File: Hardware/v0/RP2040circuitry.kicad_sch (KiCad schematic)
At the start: 29 parts, among them J1 TYPE-C-31-M-12, SW1 SW_Push, U1 RP2040, U2 NCP1117-3.3_SOT223, U3 W25Q128JVS, X1 ABM8-272-T3

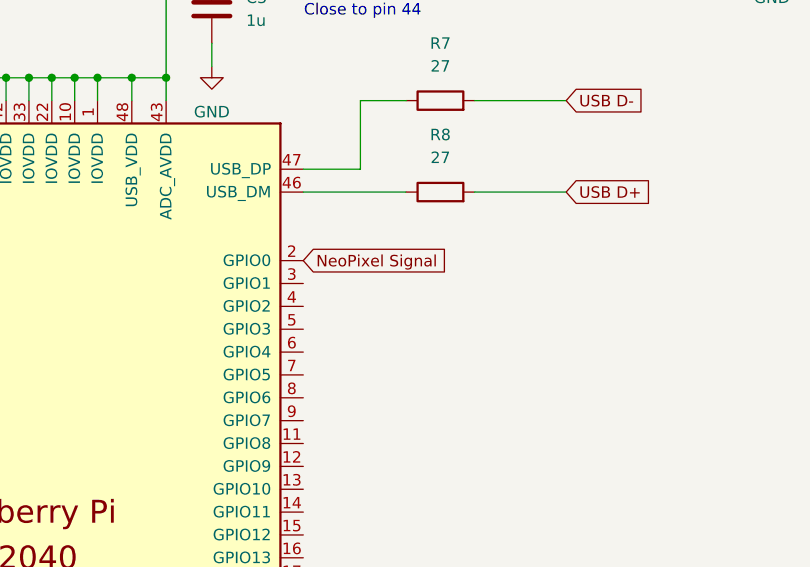
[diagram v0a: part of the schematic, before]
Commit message: he
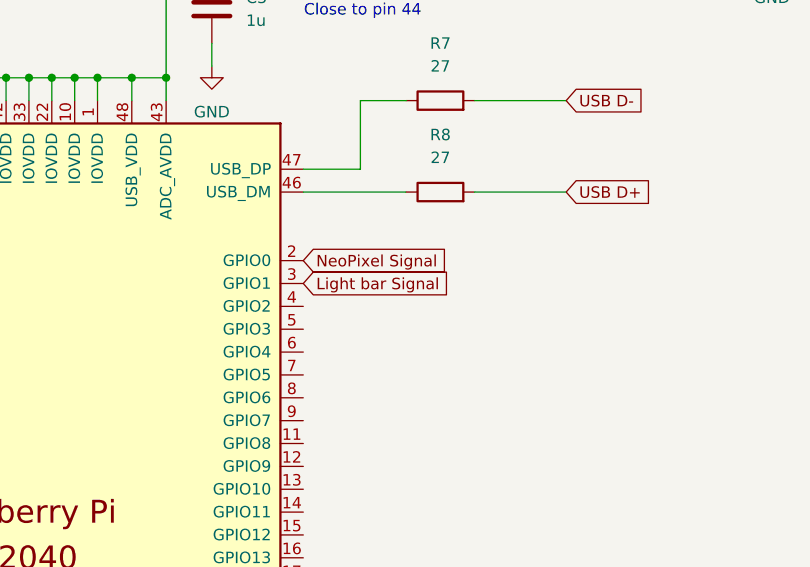
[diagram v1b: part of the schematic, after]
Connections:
- net Light bar Signal: now reaches U1.3 (GPIO1)
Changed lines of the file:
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@@
+		)
+	)
+	(global_label "Light bar Signal"
+		(shape input)
+		(at 238.76 78.74 0)
+		(fields_autoplaced yes)
+		(effects
+			(font
+				(size 1.27 1.27)
+			)
+			(justify left)
+		)
+		(property "Intersheetrefs" "${INTERSHEET_REFS}"
+			(at 257.3477 78.74 0)
+			(effects
+				(font
+					(size 1.27 1.27)
+				)
+				(justify left)
+				(hide yes)
+			)
 		)
 	)

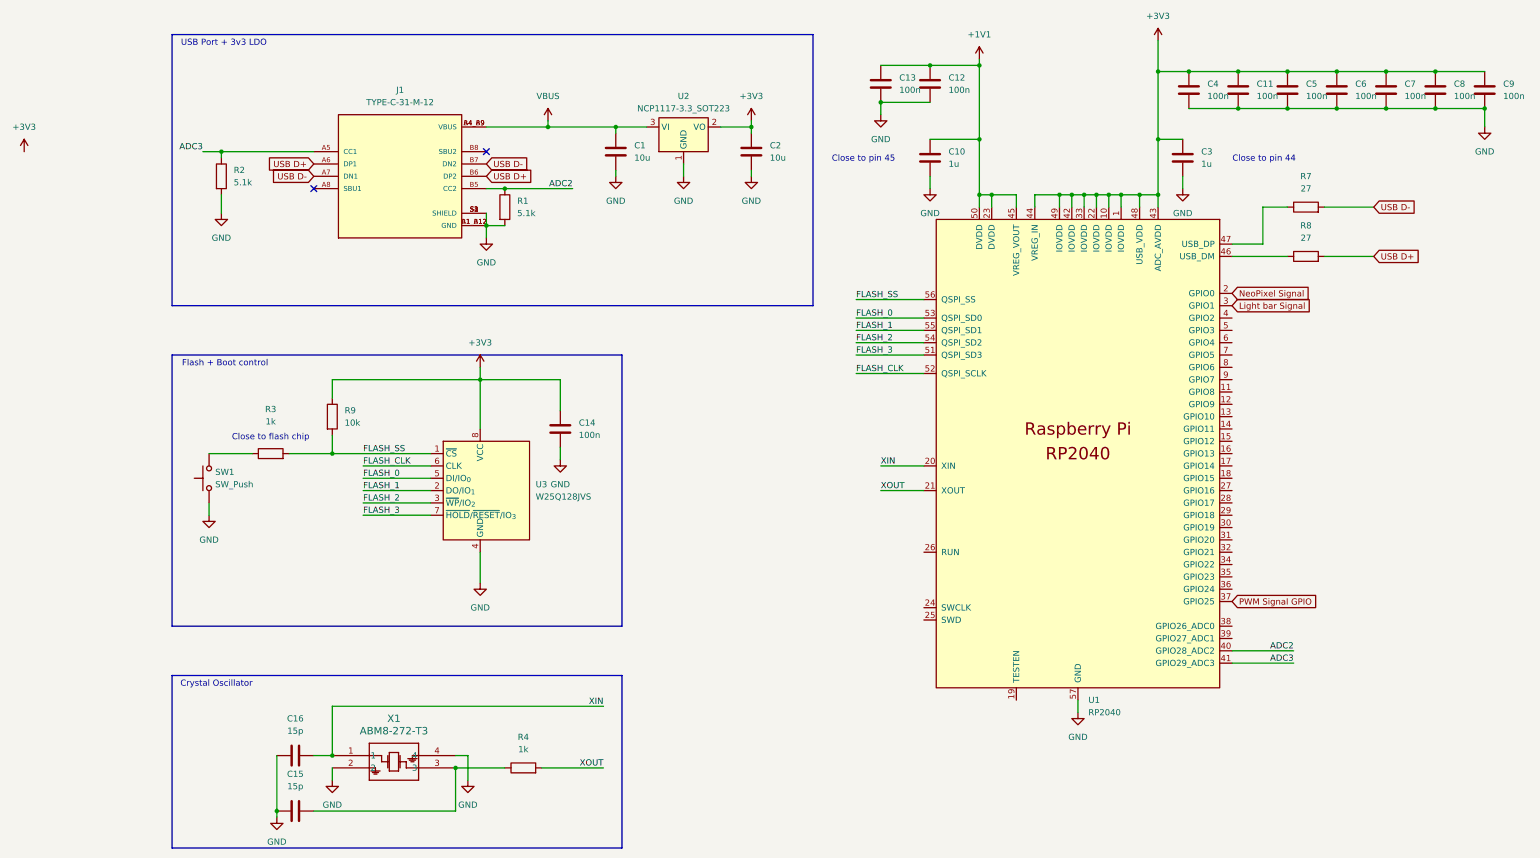
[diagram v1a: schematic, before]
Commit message: whoops i forgot to commit this
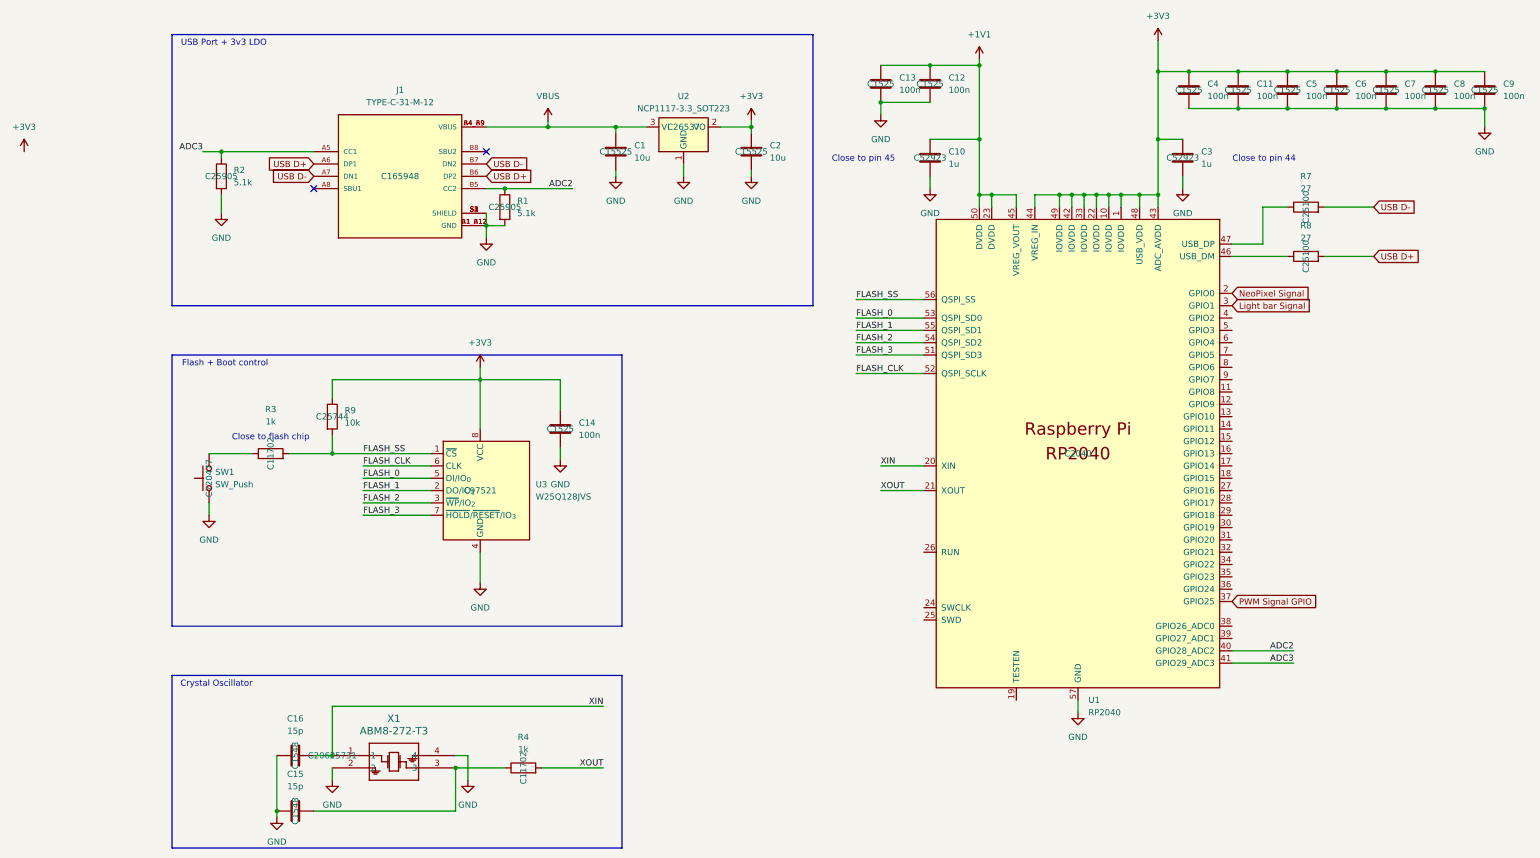
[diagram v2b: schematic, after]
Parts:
- C1, C2: LCSC (none) -> C15525
- C10, C3: LCSC (none) -> C52923
- C11, C12, C13, C14, C4, C5, C6, C7, C8, C9: LCSC (none) -> C1525
- C15, C16: LCSC (none) -> C1548
- J1: LCSC (none) -> C165948
- R1, R2: LCSC (none) -> C25905
- R3, R4: LCSC (none) -> C11702
- R7, R8: LCSC (none) -> C25100
- R9: LCSC (none) -> C25744
- SW1: LCSC (none) -> C720477
- U1: LCSC (none) -> C2040
- U2: LCSC (none) -> C26537
- U3: LCSC (none) -> C97521
- X1: LCSC (none) -> C20625731
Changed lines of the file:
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@@
 			)
 		)
+		(property "LCSC" "C1525"
+			(at 260.35 34.29 0)
+			(effects
+				(font
+					(size 1.27 1.27)
+				)
+			)
+		)
 		(pin "1"
 		)
@@
 			)
 		)
+		(property "LCSC" "C1525"
+			(at 166.37 33.02 0)
+			(effects
+				(font
+					(size 1.27 1.27)
+				)
+			)
+		)
 		(pin "1"
 		)
@@
 			)
 		)
+		(property "LCSC" "C25744"
+			(at 53.34 101.6 0)
+			(effects
+				(font
+					(size 1.27 1.27)
+				)
+			)
+		)
 		(pin "2"
 		)
@@
 			)
 		)
+		(property "LCSC" "C1525"
+			(at 280.67 34.29 0)
+			(effects
+				(font
+					(size 1.27 1.27)
+				)
+			)
+		)
 		(pin "1"
 		)
@@
 			)
 		)
+		(property "LCSC" "C1548"
+			(at 45.72 182.88 0)
+			(effects
+				(font
+					(size 1.27 1.27)
+				)
+			)
+		)
 		(pin "2"
 		)
@@
 			)
 		)
+		(property "LCSC" "C15525"
+			(at 139.7 46.99 0)
+			(effects
+				(font
+					(size 1.27 1.27)
+				)
+			)
+		)
 		(pin "2"
 		)
@@
 			)
 		)
+		(property "LCSC" "C1525"
+			(at 270.51 34.29 0)
+			(effects
+				(font
+					(size 1.27 1.27)
+				)
+			)
+		)
 		(pin "1"
 		)
@@
 			)
 		)
+		(property "LCSC" "C25100"
+			(at 254 68.58 0)
+			(effects
+				(font
+					(size 1.27 1.27)
+				)
+			)
+		)
 		(pin "2"
 		)
@@
 			)
 		)
+		(property "LCSC" "C11702"
+			(at 40.64 109.22 0)
+			(effects
+				(font
+					(size 1.27 1.27)
+				)
+			)
+		)
 		(pin "2"
 		)
@@
 			)
 		)
+		(property "LCSC" "C1525"
+			(at 290.83 34.29 0)
+			(effects
+				(font
+					(size 1.27 1.27)
+				)
+			)
+		)
 		(pin "1"
 		)
@@
 			)
 		)
+		(property "LCSC" "C1525"
+			(at 100.33 104.14 0)
+			(effects
+				(font
+					(size 1.27 1.27)
+				)
+			)
+		)
 		(pin "1"
 		)
@@
 			)
 		)
+		(property "LCSC" "C720477"
+			(at 27.94 114.3 0)
+			(effects
+				(font
+					(size 1.27 1.27)
+				)
+			)
+		)
 		(pin "1"
 		)
@@
 			)
 		)
+		(property "LCSC" "C26537"
+			(at 125.73 41.91 0)
+			(effects
+				(font
+					(size 1.27 1.27)
+				)
+			)
+		)
 		(pin "3"
 		)
@@
 			)
 		)
+		(property "LCSC" "C1525"
+			(at 250.19 34.29 0)
+			(effects
+				(font
+					(size 1.27 1.27)
+				)
+			)
+		)
 		(pin "1"
 		)
@@
 			)
 		)
+		(property "LCSC" "C15525"
+			(at 111.76 46.99 0)
+			(effects
+				(font
+					(size 1.27 1.27)
+				)
+			)
+		)
 		(pin "2"
 		)
@@
 			)
 		)
+		(property "LCSC" "C25905"
+			(at 30.48 52.07 0)
+			(effects
+				(font
+					(size 1.27 1.27)
+				)
+			)
+		)
 		(pin "2"
 		)
@@
 			)
 		)
+		(property "LCSC" "C11702"
+			(at 92.71 173.99 0)
+			(effects
+				(font
+					(size 1.27 1.27)
+				)
+			)
+		)
 		(pin "2"
 		)
@@
 			)
 		)
+		(property "LCSC" "C1525"
+			(at 229.87 34.29 0)
+			(effects
+				(font
+					(size 1.27 1.27)
+				)
+			)
+		)
 		(pin "1"
 		)
@@
 			)
 		)
+		(property "LCSC" "C1525"
+			(at 240.03 34.29 0)
+			(effects
+				(font
+					(size 1.27 1.27)
+				)
+			)
+		)
 		(pin "1"
 		)
@@
 			)
 		)
+		(property "LCSC" "C2040"
+			(at 207.01 109.22 0)
+			(effects
+				(font
+					(size 1.27 1.27)
+				)
+			)
+		)
 		(pin "7"
 		)
@@
 			)
 		)
+		(property "LCSC" "C1548"
+			(at 45.72 171.45 0)
+			(effects
+				(font
+					(size 1.27 1.27)
+				)
+			)
+		)
 		(pin "2"
 		)
@@
 			)
 		)
+		(property "LCSC" "C25905"
+			(at 88.9 58.42 0)
+			(effects
+				(font
+					(size 1.27 1.27)
+				)
+			)
+		)
 		(pin "2"
 		)
@@
 			)
 		)
+		(property "LCSC" "C52923"
+			(at 228.6 48.26 0)
+			(effects
+				(font
+					(size 1.27 1.27)
+				)
+			)
+		)
 		(pin "1"
 		)
@@
 			)
 		)
+		(property "LCSC" "C97521"
+			(at 83.82 116.84 0)
+			(effects
+				(font
+					(size 1.27 1.27)
+				)
+			)
+		)
 		(pin "1"
 		)
@@
 			)
 		)
+		(property "LCSC" "C52923"
+			(at 176.53 48.26 0)
+			(effects
+				(font
+					(size 1.27 1.27)
+				)
+			)
+		)
 		(pin "1"
 		)
@@
 			)
 		)
+		(property "LCSC" "C1525"
+			(at 176.53 33.02 0)
+			(effects
+				(font
+					(size 1.27 1.27)
+				)
+			)
+		)
 		(pin "1"
 		)
@@
 			)
 		)
+		(property "LCSC" "C25100"
+			(at 254 58.42 0)
+			(effects
+				(font
+					(size 1.27 1.27)
+				)
+			)
+		)
 		(pin "2"
 		)
@@
 			)
 		)
+		(property "LCSC" "C165948"
+			(at 67.31 52.07 0)
+			(effects
+				(font
+					(size 1.27 1.27)
+				)
+			)
+		)
 		(pin "B1_A12"
 		)
@@
 			)
 		)
+		(property "LCSC" "C20625731"
+			(at 53.34 171.45 0)
+			(effects
+				(font
+					(size 1.27 1.27)
+				)
+			)
+		)
